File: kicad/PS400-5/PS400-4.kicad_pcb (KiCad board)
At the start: 2 copper layers, 13.5 x 13.1 mm, 28 parts, among them J1 Conn, J2 Conn, J3 Conn, J4 Conn, J5 Conn, Q1 RUM002N05, Q2 Q_NPN_BEC, Q3 RUM002N05, T1 B82801A150, U2 PIC10F206-IOT

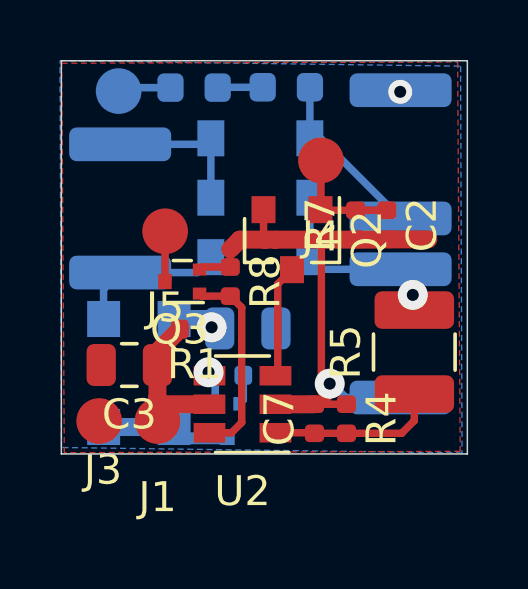
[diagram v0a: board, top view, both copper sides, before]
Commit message: изменено:      Documents/circuit.png 	изменено:      kicad/PS400-5/PS400-4.kicad_pcb 	изменено:      kicad/PS400-5/PS400-4.kicad_pcb-bak 	изменено:      kicad/PS400-5/PS400-4.pdf 	изменено:      kicad/PS400-5/PS400-4.sch 	изменено:      kicad/PS400-5/PS400-4.sch-bak
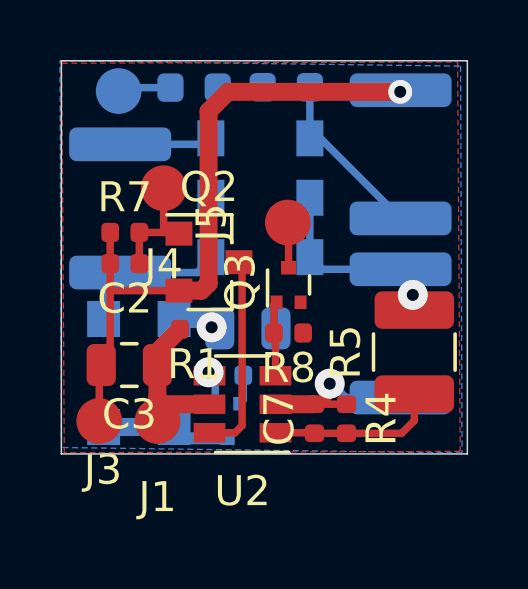
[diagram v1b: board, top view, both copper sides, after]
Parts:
- moved C2 8.83 mm to (33.9, 49.4), turned to 180 degrees
- moved R7 7.70 mm to (33.9, 48.3), turned to 0 degrees
- moved J4 5.33 mm to (35.2, 46.9)
- moved J5 4.10 mm to (39.3, 48.0), turned to 270 degrees
- moved Q3 3.55 mm to (39.3, 50.1), turned to 90 degrees
- moved Q2 2.87 mm to (36.7, 49.3), turned to 0 degrees
- moved R8 2.59 mm to (39.3, 51.7), turned to 180 degrees
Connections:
- U2 pad 3: Net-(Q2-Pad3) -> Net-(Q3-Pad1)
- U2 pad 6: Net-(Q3-Pad1) -> Net-(Q2-Pad3)
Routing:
- net GND: track 21.4 -> 29.3 mm
- net Net-(Q3-Pad1): track 6.65 -> 2.51 mm
- net Net-(Q2-Pad3): track 3.76 -> 6.68 mm
